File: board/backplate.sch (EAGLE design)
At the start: 22 parts, among them IC1 MAX7219CNG, IC2 MAX7219CNG, IC3 MAX7219CNG, IC4 MAX7219CNG

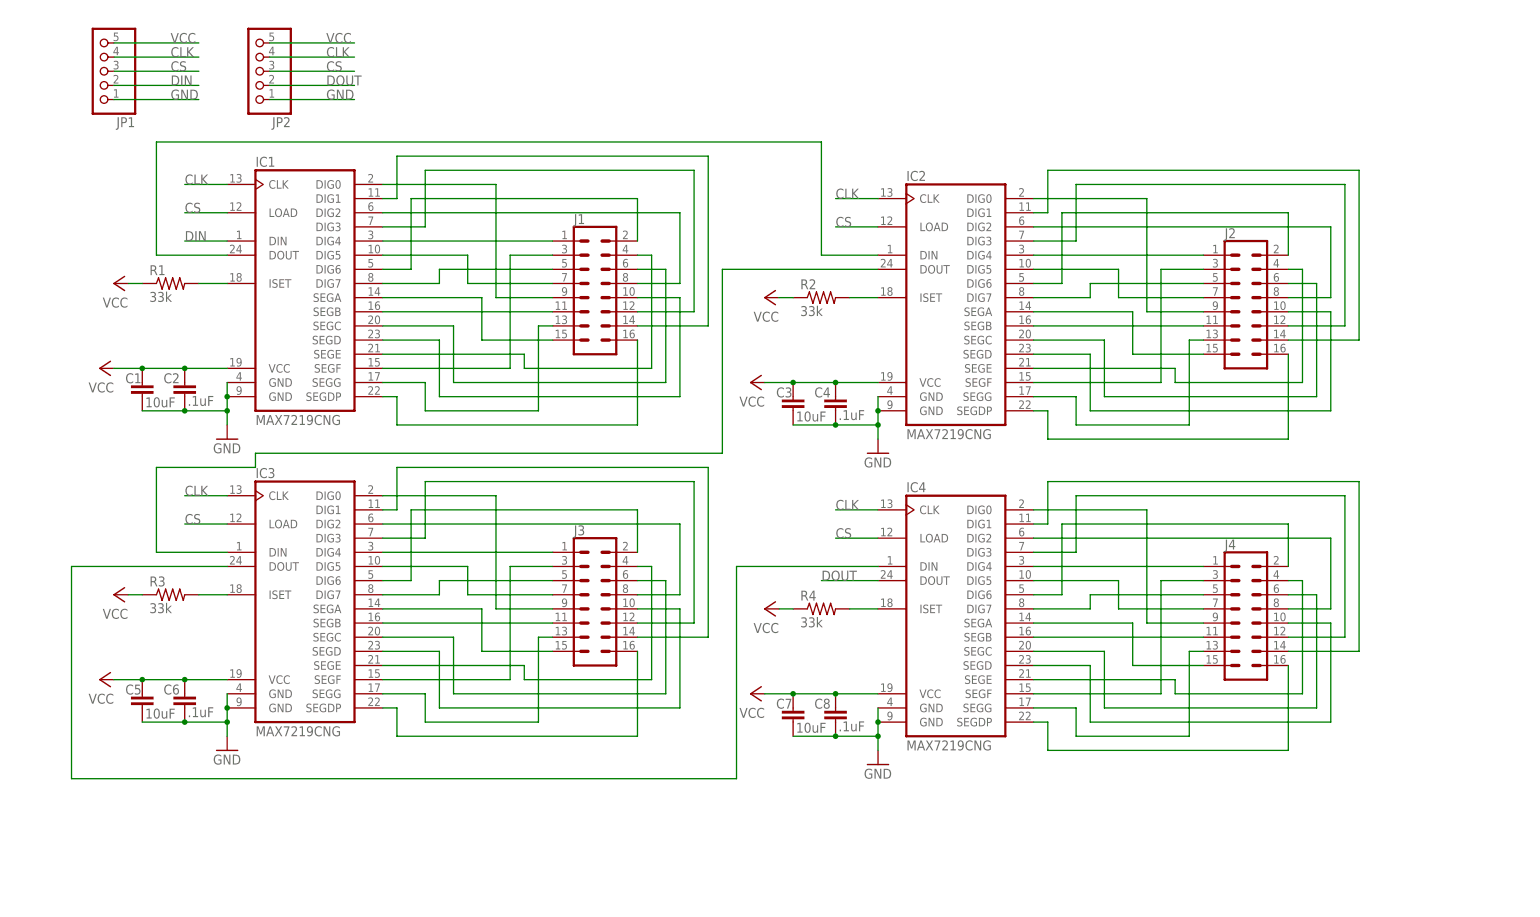
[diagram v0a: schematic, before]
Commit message: backplight v2
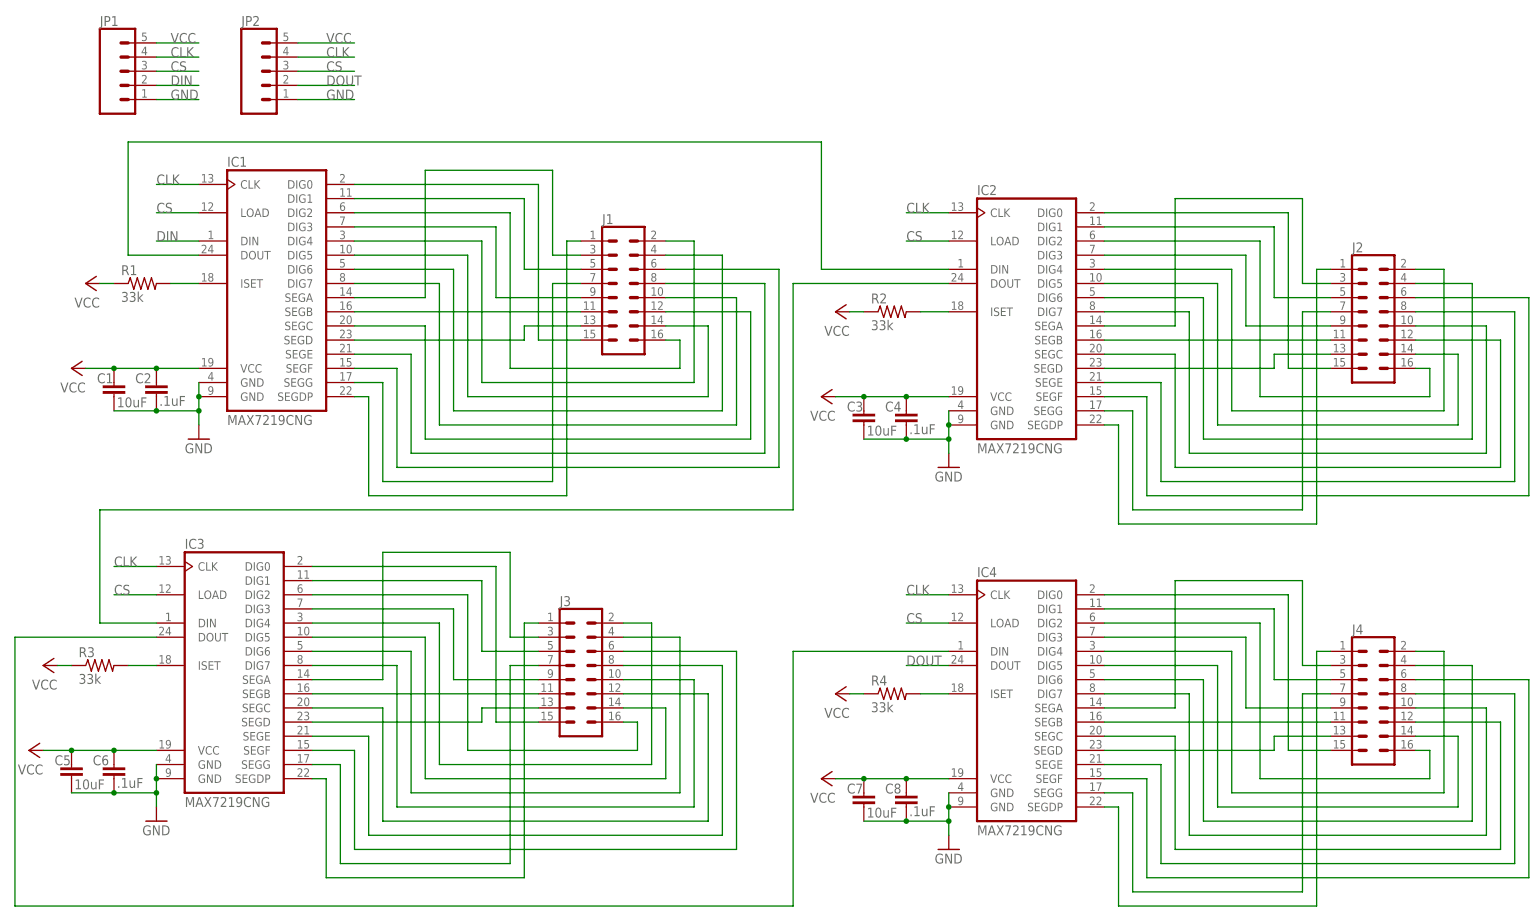
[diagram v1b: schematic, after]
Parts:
- JP1, JP2: device pinhead:PINHD-1X55X2MM -> SparkFun-Connectors:CONN_05
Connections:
- removed net N$13 (its old number): IC1.DIG3, J1.12
- removed net N$17: IC1.SEGA, J1.15
- removed net N$19 (its old number): IC2.DIG4, J2.1
- removed net N$20 (its old number): IC2.DIG6, J2.2
- removed net N$29: IC2.DIG3, J2.12
- removed net N$31: IC2.DIG1, J2.14
- removed net N$33 (its old number): IC2.SEGA, J2.15
- removed net N$34: IC2.DIG2, J2.8
- removed net N$40 (its old number): IC3.DIG7, J3.5
- removed net N$41 (its old number): IC3.SEGC, J3.6
- removed net N$58 (its old number): IC4.SEGC, J4.6
- removed net N$59 (its old number): IC4.DIG5, J4.7
- removed net N$63: IC4.DIG3, J4.12
- removed net N$65: IC4.DIG1, J4.14
- removed net N$68: IC4.DIG2, J4.8
- new net N$2: IC1.SEGD, J1.13
- new net N$28: IC2.DIG6, J2.4
- new net N$35: IC2.SEGD, J2.13
- new net N$45: IC3.DIG2, J3.16
- new net N$62: IC4.DIG1, J4.5
- new net N$69: IC4.DIG5, J4.14
- new net N$71: IC1.SEGC, J1.12
- new net N$72: IC4.DIG6, J4.4
- new net N$73: IC4.DIG7, J4.10
- new net N$74: IC4.SEGA, J4.3
- new net N$76: IC4.SEGD, J4.13
- new net N$77: IC4.SEGE, J4.8
- new net N$78: IC4.SEGF, J4.6
- new net N$79: IC4.SEGG, J4.7
- new net N$80: IC4.SEGDP, J4.1
- net N$10: now also IC1.DIG7; no longer IC1.SEGD
- net N$11: now also IC1.SEGA, J1.3; no longer IC1.DIG0, J1.9
- net N$14: now also IC1.SEGE, J1.8; no longer IC1.SEGG, J1.13
- net N$15: now also IC1.SEGF, J1.6; no longer IC1.DIG1, J1.14
- net N$16: now also IC1.SEGG, J1.7; no longer IC1.SEGDP, J1.16
- net N$18: now also IC1.SEGDP, J1.1; no longer IC1.DIG2, J1.8
- net N$21: now also IC2.SEGC, J2.12; no longer IC2.SEGF, J2.3
- net N$22: now also IC2.DIG0, J2.15; no longer IC2.SEGE, J2.4
- net N$23: now also IC2.DIG1; no longer IC2.DIG7
- net N$24: now also IC2.DIG2, J2.16; no longer IC2.SEGC, J2.6
- net N$25: now also IC2.DIG3, J2.9; no longer IC2.DIG5, J2.7
- net N$26: now also IC2.DIG4, J2.2; no longer IC2.SEGD, J2.10
- net N$27: now also IC2.DIG5, J2.14; no longer IC2.DIG0, J2.9
- net N$3: now also IC1.DIG0, J1.15; no longer IC1.DIG4, J1.1
- net N$30: now also IC2.DIG7, J2.10; no longer IC2.SEGG, J2.13
- net N$32: now also IC2.SEGA, J2.3; no longer IC2.SEGDP, J2.16
- net N$36: now also IC2.SEGE, J2.8; no longer IC3.DIG4, J3.1
- net N$37: now also IC2.SEGF, J2.6; no longer IC3.DIG6, J3.2
- net N$38: now also IC2.SEGG, J2.7; no longer IC3.SEGF, J3.3
- net N$39: now also IC2.SEGDP, J2.1; no longer IC3.SEGE, J3.4
- net N$4: now also IC1.DIG1, J1.5; no longer IC1.DIG6, J1.2
- net N$42: now also IC3.SEGC, J3.12; no longer IC3.DIG5, J3.7
- net N$43: now also IC3.DIG0, J3.15; no longer IC3.SEGD, J3.10
- net N$44: now also IC3.DIG1, J3.5; no longer IC3.DIG0, J3.9
- net N$46: now also J3.9; no longer J3.12
- net N$47: now also IC3.DIG4, J3.2; no longer IC3.SEGG, J3.13
- net N$48: now also IC3.DIG5; no longer IC3.DIG1
- net N$49: now also IC3.DIG6, J3.4; no longer IC3.SEGDP, J3.16
- net N$5: now also IC1.DIG2, J1.16; no longer IC1.SEGF, J1.3
- net N$50: now also IC3.DIG7, J3.10; no longer IC3.SEGA, J3.15
- net N$51: now also IC3.SEGA, J3.3; no longer IC3.DIG2, J3.8
- net N$53: now also IC3.SEGD, J3.13; no longer IC4.DIG4, J4.1
- net N$54: now also IC3.SEGE, J3.8; no longer IC4.DIG6, J4.2
- net N$55: now also IC3.SEGF, J3.6; no longer IC4.SEGF, J4.3
- net N$56: now also IC3.SEGG, J3.7; no longer IC4.SEGE, J4.4
- net N$57: now also IC3.SEGDP, J3.1; no longer IC4.DIG7, J4.5
- net N$6: now also IC1.DIG3, J1.9; no longer IC1.SEGE, J1.4
- net N$60: now also IC4.SEGC, J4.12; no longer IC4.SEGD, J4.10
- net N$61: now also J4.15; no longer J4.9
- net N$64: now also IC4.DIG2, J4.16; no longer IC4.SEGG, J4.13
- net N$66: now also IC4.DIG3, J4.9; no longer IC4.SEGDP, J4.16
- net N$67: now also IC4.DIG4, J4.2; no longer IC4.SEGA, J4.15
- net N$7: now also IC1.DIG4, J1.2; no longer IC1.DIG7, J1.5
- net N$8: now also IC1.DIG5, J1.14; no longer IC1.SEGC, J1.6
- net N$9: now also IC1.DIG6, J1.4; no longer IC1.DIG5, J1.7
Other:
- note removed: "https://i.imgur.com/5x2sXNw.png pins"
- moved on the sheet: C1, C2, C3, C4, C5, C6, C7, C8, IC1, IC2, IC3, IC4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

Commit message: based on https://i.imgur.com/TE96g29.png" "
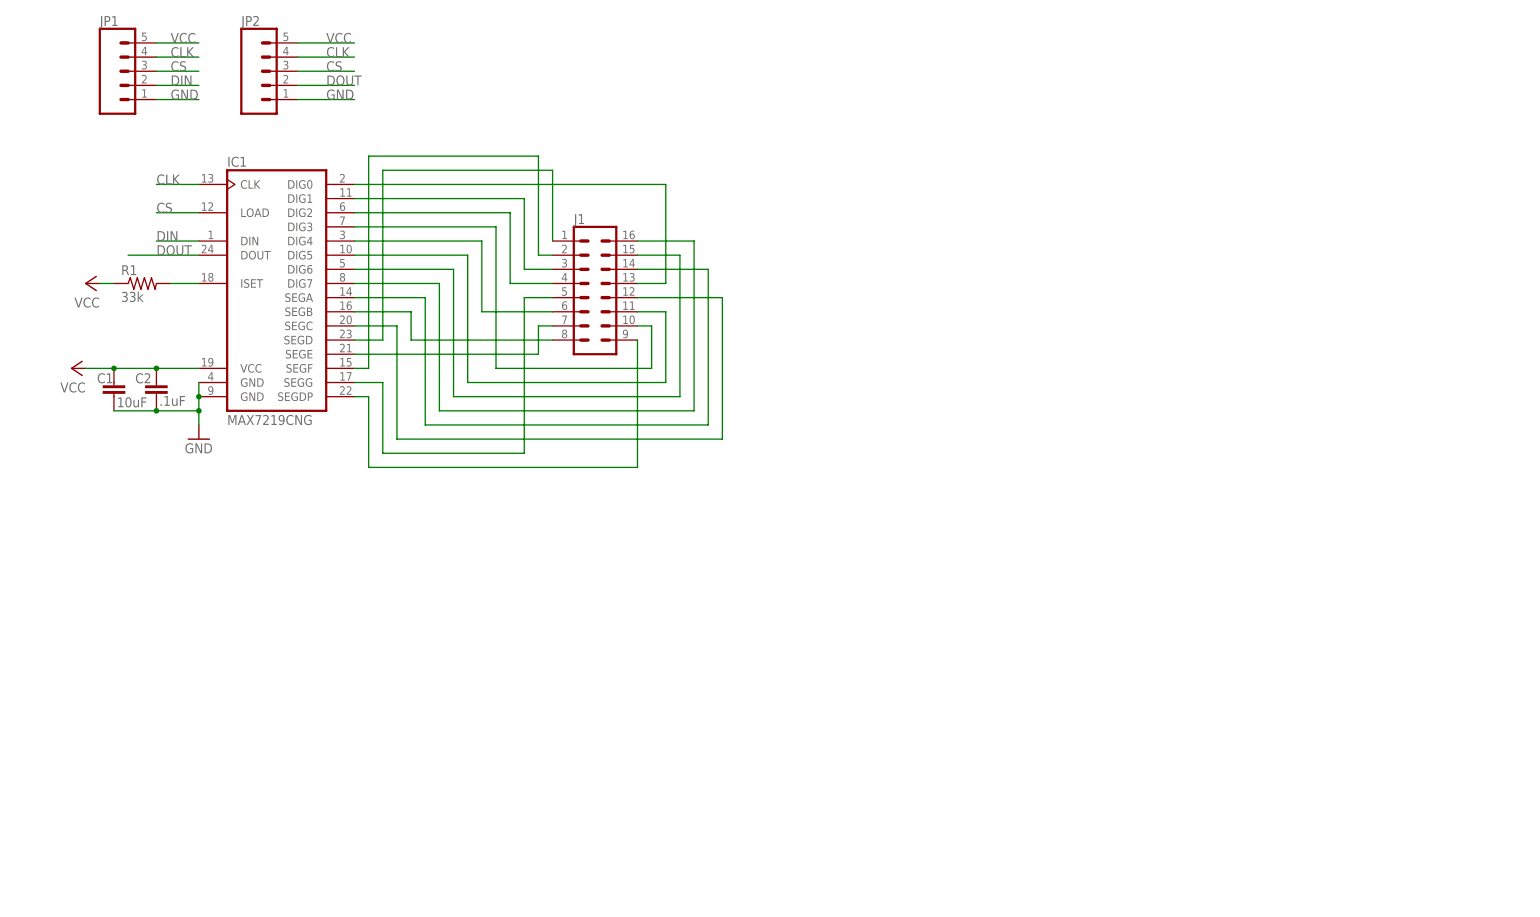
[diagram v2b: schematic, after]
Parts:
- removed C3, C5, C7: 10uF, TinyTony_ShenzenReady:CAP0805
- removed C4, C6, C8: .1uF, TinyTony_ShenzenReady:CAP0805
- removed IC2, IC3, IC4: MAX7219CNG, maxim:MAX7219CNG
- removed J2, J3, J4: (no value), SparkFun-Connectors:CONN_08X2
- removed R2, R3, R4: 33k, rcl:R-US_V526-0
- J1: device SparkFun-Connectors:CONN_08X2 -> backplate:CONN_08X2IC
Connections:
- removed net N$18: IC1.SEGDP, J1.1
- removed net N$19: IC2.ISET, R2.2
- removed net N$20: IC2.DOUT, IC3.DIN
- removed net N$21: IC2.SEGC, J2.12
- removed net N$22: IC2.DIG0, J2.15
- removed net N$23: IC2.DIG1, J2.5
- removed net N$24: IC2.DIG2, J2.16
- removed net N$25: IC2.DIG3, J2.9
- removed net N$26: IC2.DIG4, J2.2
- removed net N$27: IC2.DIG5, J2.14
- removed net N$28: IC2.DIG6, J2.4
- removed net N$3 (its old number): IC1.DIG0, J1.15
- removed net N$30: IC2.DIG7, J2.10
- removed net N$32: IC2.SEGA, J2.3
- removed net N$33: IC2.SEGB, J2.11
- removed net N$35: IC2.SEGD, J2.13
- removed net N$36: IC2.SEGE, J2.8
- removed net N$37: IC2.SEGF, J2.6
- removed net N$38: IC2.SEGG, J2.7
- removed net N$39: IC2.SEGDP, J2.1
- removed net N$40: IC3.ISET, R3.2
- removed net N$41: IC1.DOUT, IC2.DIN
- removed net N$42: IC3.SEGC, J3.12
- removed net N$43: IC3.DIG0, J3.15
- removed net N$44: IC3.DIG1, J3.5
- removed net N$45: IC3.DIG2, J3.16
- removed net N$46: IC3.DIG3, J3.9
- removed net N$47: IC3.DIG4, J3.2
- removed net N$48: IC3.DIG5, J3.14
- removed net N$49: IC3.DIG6, J3.4
- removed net N$50: IC3.DIG7, J3.10
- removed net N$51: IC3.SEGA, J3.3
- removed net N$52: IC3.SEGB, J3.11
- removed net N$53: IC3.SEGD, J3.13
- removed net N$54: IC3.SEGE, J3.8
- removed net N$55: IC3.SEGF, J3.6
- removed net N$56: IC3.SEGG, J3.7
- removed net N$57: IC3.SEGDP, J3.1
- removed net N$58: IC4.ISET, R4.2
- removed net N$59: IC3.DOUT, IC4.DIN
- removed net N$60: IC4.SEGC, J4.12
- removed net N$61: IC4.DIG0, J4.15
- removed net N$62: IC4.DIG1, J4.5
- removed net N$64: IC4.DIG2, J4.16
- removed net N$66: IC4.DIG3, J4.9
- removed net N$67: IC4.DIG4, J4.2
- removed net N$69: IC4.DIG5, J4.14
- removed net N$71: IC1.SEGC, J1.12
- removed net N$72: IC4.DIG6, J4.4
- removed net N$73: IC4.DIG7, J4.10
- removed net N$74: IC4.SEGA, J4.3
- removed net N$75: IC4.SEGB, J4.11
- removed net N$76: IC4.SEGD, J4.13
- removed net N$77: IC4.SEGE, J4.8
- removed net N$78: IC4.SEGF, J4.6
- removed net N$79: IC4.SEGG, J4.7
- removed net N$8 (its old number): IC1.DIG5, J1.14
- removed net N$80: IC4.SEGDP, J4.1
- new net N$12: IC1.SEGC, J1.10
- new net N$17: IC1.SEGDP, J1.16
- new net N$4: IC1.DIG2, J1.7
- new net N$9: IC1.DIG7, J1.2
- net CLK: no longer IC2.CLK, IC3.CLK, IC4.CLK
- net CS: no longer IC2.LOAD, IC3.LOAD, IC4.LOAD
- net DOUT: now also IC1.DOUT; no longer IC4.DOUT
- net GND: no longer C3.2, C4.2, C5.2, C6.2, C7.2, C8.2, IC2.GND@1, IC2.GND@2, IC3.GND@1, IC3.GND@2, IC4.GND@1, IC4.GND@2
- net N$10: now also IC1.SEGA, J1.6; no longer IC1.DIG7, J1.10
- net N$11: now also IC1.SEGB, J1.15; no longer IC1.SEGA, J1.3
- net N$13: now also IC1.SEGD, J1.1; no longer IC1.SEGB, J1.11
- net N$14: now also J1.13; no longer J1.8
- net N$15: now also J1.3; no longer J1.6
- net N$16: now also J1.9; no longer J1.7
- net N$2: now also IC1.DIG0, J1.8; no longer IC1.SEGD, J1.13
- net N$5: now also IC1.DIG3, J1.14; no longer IC1.DIG2, J1.16
- net N$6: now also IC1.DIG4, J1.11; no longer IC1.DIG3, J1.9
- net N$7: now also IC1.DIG5, J1.12; no longer IC1.DIG4, J1.2
- net VCC: no longer C3.1, C4.1, C5.1, C6.1, C7.1, C8.1, IC2.VCC, IC3.VCC, IC4.VCC, R2.1, R3.1, R4.1
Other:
- moved on the sheet: J1

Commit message: routed 4
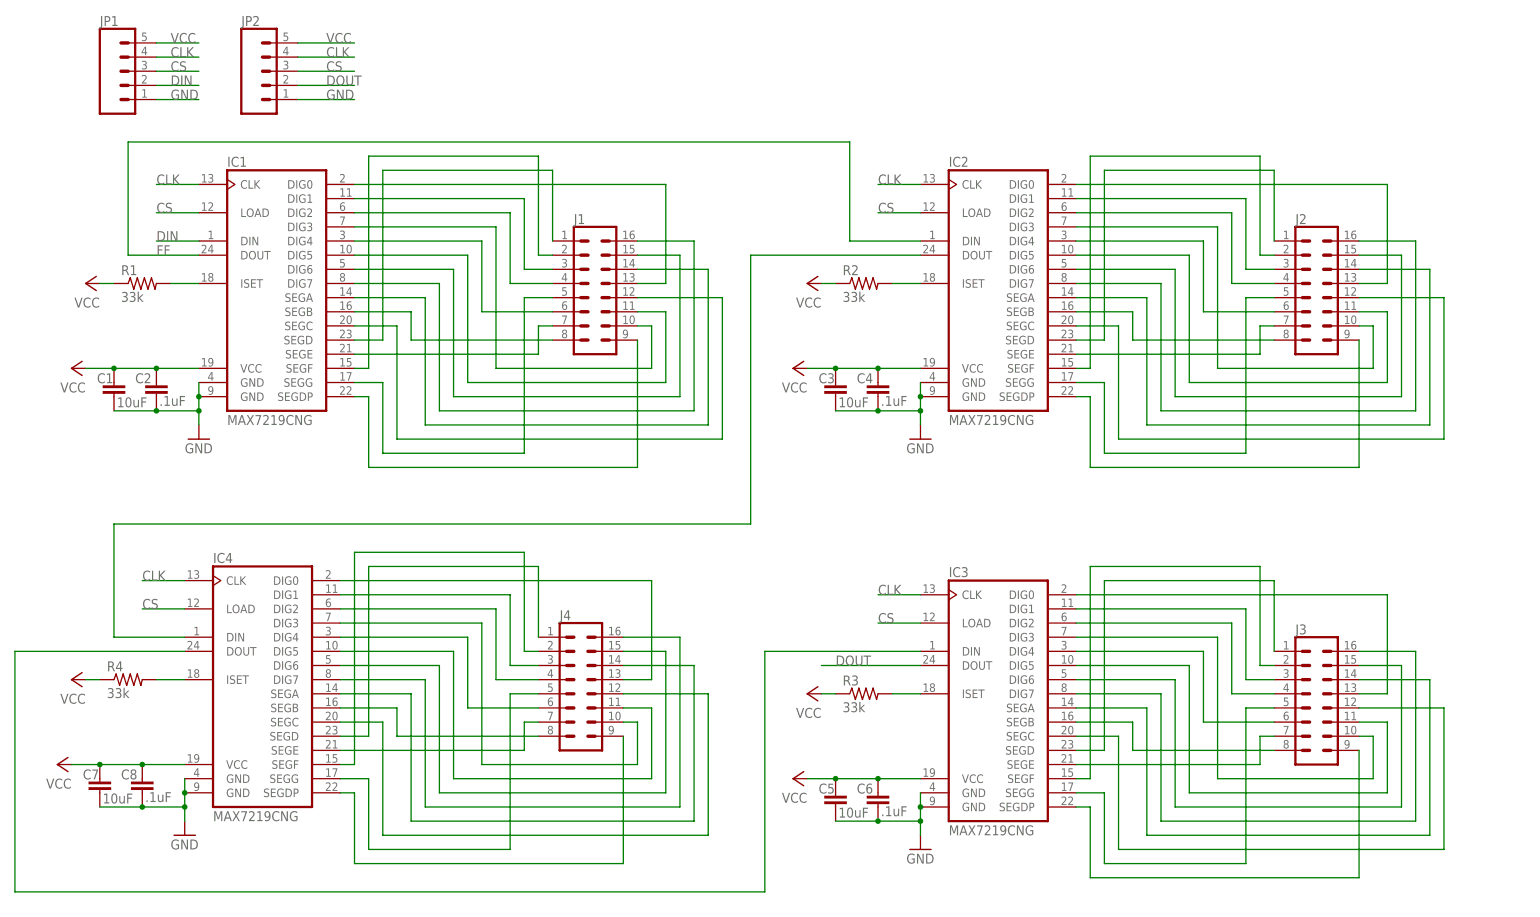
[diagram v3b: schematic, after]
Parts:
- added C3, C5, C7: 10uF, TinyTony_ShenzenReady:CAP0805
- added C4, C6, C8: .1uF, TinyTony_ShenzenReady:CAP0805
- added IC2, IC3, IC4: MAX7219CNG, maxim:MAX7219CNG
- added J2, J3, J4: (no value), backplate:CONN_08X2IC
- added R2, R3, R4: 33k, rcl:R-US_V526-0
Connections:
- new net FF: IC1.DOUT, IC2.DIN
- new net N$18: IC2.ISET, R2.2
- new net N$19: IC2.DIG0, J2.8
- new net N$20: IC2.DIG1, J2.5
- new net N$21: IC2.DIG2, J2.7
- new net N$22: IC2.DIG3, J2.14
- new net N$23: IC2.DIG4, J2.11
- new net N$24: IC2.DIG5, J2.12
- new net N$25: IC2.DIG6, J2.4
- new net N$26: IC2.DIG7, J2.2
- new net N$27: IC2.SEGA, J2.6
- new net N$28: IC2.SEGB, J2.15
- new net N$29: IC2.SEGC, J2.10
- new net N$30: IC2.SEGD, J2.1
- new net N$31: IC2.SEGE, J2.13
- new net N$32: IC2.SEGF, J2.3
- new net N$33: IC2.SEGG, J2.9
- new net N$34: IC2.SEGDP, J2.16
- new net N$35: IC3.ISET, R3.2
- new net N$36: IC3.DIG0, J3.8
- new net N$37: IC3.DIG1, J3.5
- new net N$38: IC3.DIG2, J3.7
- new net N$39: IC3.DIG3, J3.14
- new net N$40: IC3.DIG4, J3.11
- new net N$41: IC3.DIG5, J3.12
- new net N$42: IC3.DIG6, J3.4
- new net N$43: IC3.DIG7, J3.2
- new net N$44: IC3.SEGA, J3.6
- new net N$45: IC3.SEGB, J3.15
- new net N$46: IC3.SEGC, J3.10
- new net N$47: IC3.SEGD, J3.1
- new net N$48: IC3.SEGE, J3.13
- new net N$49: IC3.SEGF, J3.3
- new net N$50: IC3.SEGG, J3.9
- new net N$51: IC3.SEGDP, J3.16
- new net N$52: IC4.ISET, R4.2
- new net N$53: IC4.DIG0, J4.8
- new net N$54: IC4.DIG1, J4.5
- new net N$55: IC4.DIG2, J4.7
- new net N$56: IC4.DIG3, J4.14
- new net N$57: IC4.DIG4, J4.11
- new net N$58: IC4.DIG5, J4.12
- new net N$59: IC4.DIG6, J4.4
- new net N$60: IC4.DIG7, J4.2
- new net N$61: IC4.SEGA, J4.6
- new net N$62: IC4.SEGB, J4.15
- new net N$63: IC4.SEGC, J4.10
- new net N$64: IC4.SEGD, J4.1
- new net N$65: IC4.SEGE, J4.13
- new net N$66: IC4.SEGF, J4.3
- new net N$67: IC4.SEGG, J4.9
- new net N$68: IC4.SEGDP, J4.16
- new net N$69: IC2.DOUT, IC4.DIN
- new net N$70: IC3.DIN, IC4.DOUT
- net CLK: now also IC2.CLK, IC3.CLK, IC4.CLK
- net CS: now also IC2.LOAD, IC3.LOAD, IC4.LOAD
- net DOUT: now also IC3.DOUT; no longer IC1.DOUT
- net GND: now also C3.2, C4.2, C5.2, C6.2, C7.2, C8.2, IC2.GND@1, IC2.GND@2, IC3.GND@1, IC3.GND@2, IC4.GND@1, IC4.GND@2
- net VCC: now also C3.1, C4.1, C5.1, C6.1, C7.1, C8.1, IC2.VCC, IC3.VCC, IC4.VCC, R2.1, R3.1, R4.1
